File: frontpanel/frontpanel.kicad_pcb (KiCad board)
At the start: 2 copper layers, 20 x 128.5 mm, 1 part

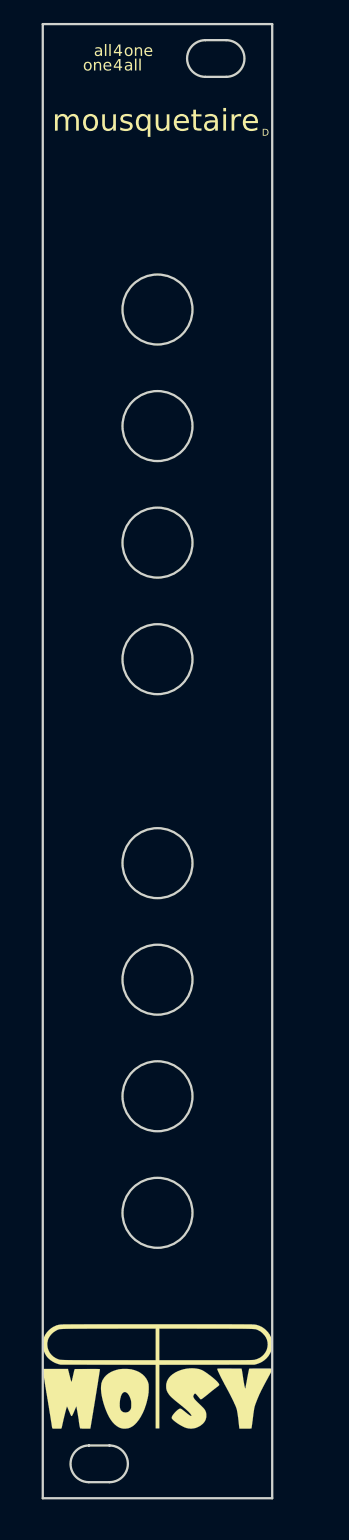
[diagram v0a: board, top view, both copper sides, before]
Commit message: :sparkles: Add design for both module variants
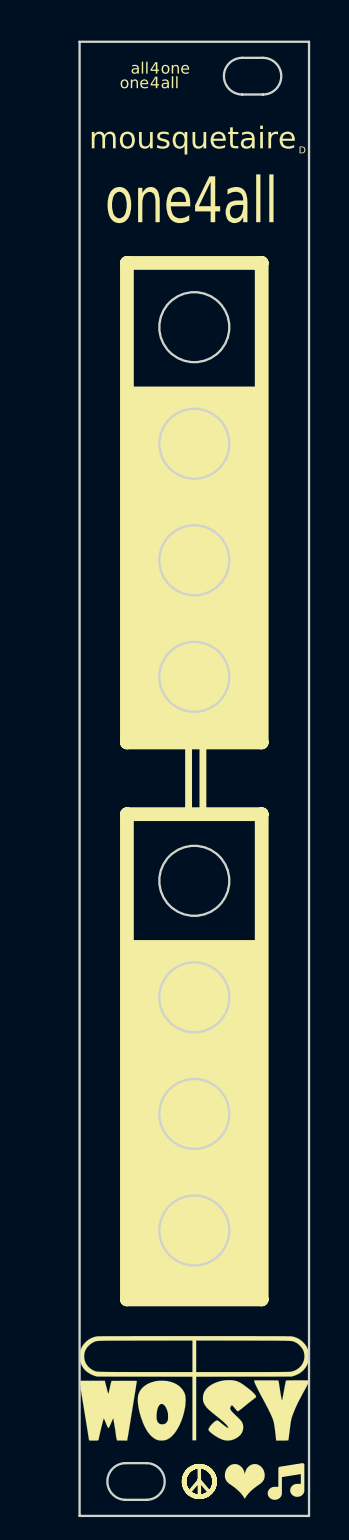
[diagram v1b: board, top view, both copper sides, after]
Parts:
- added Ref**: Val**, moPsy_KiCad:moPsy_logo_kicad_20x09_FSilk, B.Cu at (140.0, 157.5)
- moved Ref** 3.37 mm to (140.0, 157.5)
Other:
- outline, holes or cut-outs redrawn
- board text added: "all4one"
- board text added: "one4all"
- board text removed: "Peace Love Music"
